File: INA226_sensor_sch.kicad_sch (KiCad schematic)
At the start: 6 parts, among them U7 INA226AIDGSR, U8 INA226AIDGSR

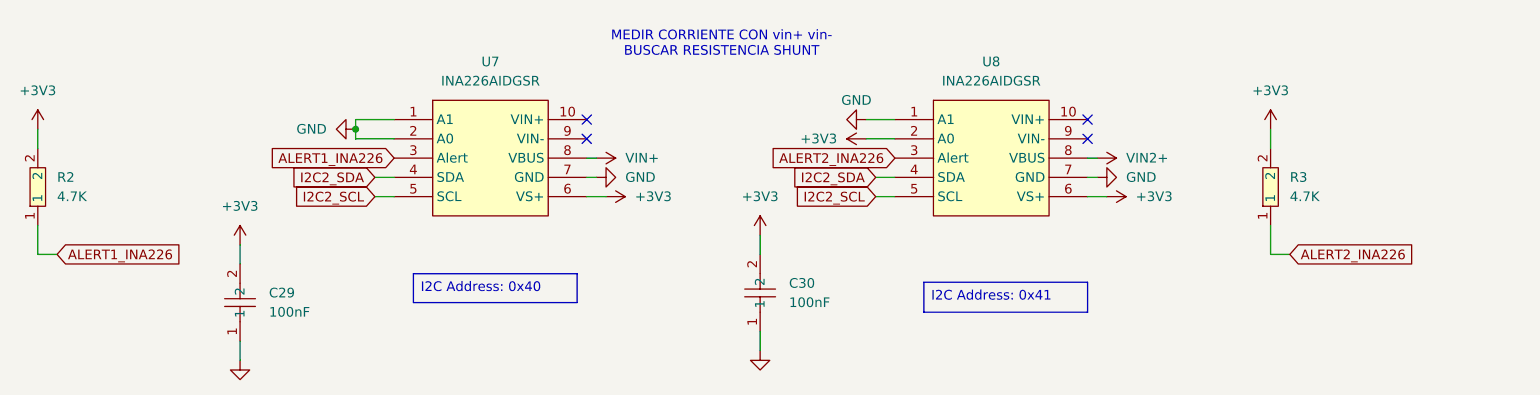
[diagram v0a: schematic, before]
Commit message: BECERRA
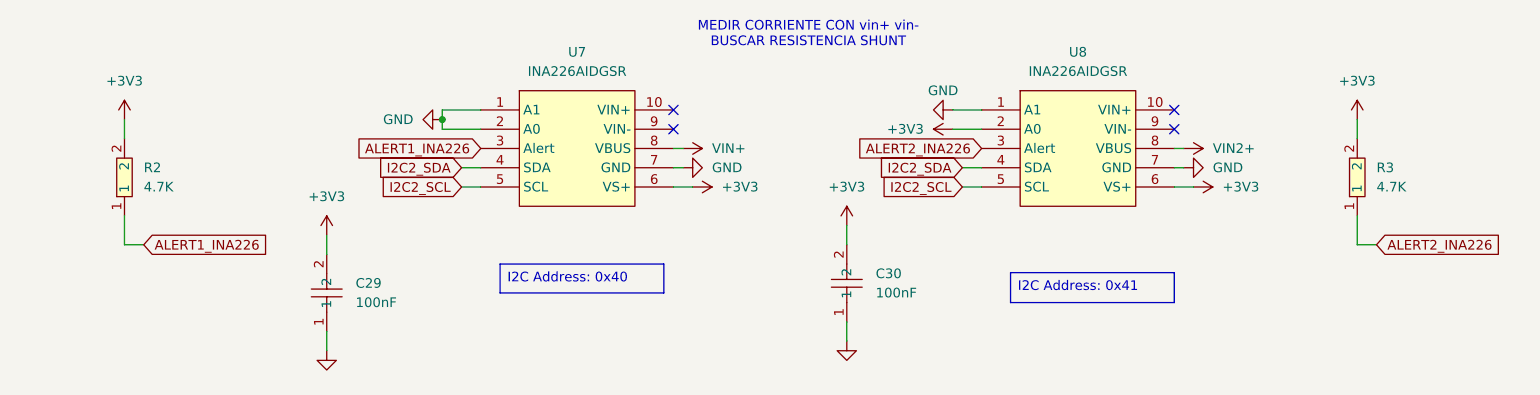
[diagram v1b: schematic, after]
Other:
- moved on the sheet: C29, C30, R2, R3, U7, U8
